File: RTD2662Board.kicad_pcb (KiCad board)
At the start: 2 copper layers, 100 x 70 mm, 263 parts, among them J1 DVI, J10 UART/I2C, J11 LCD Connector, J12 SPDIFF, J13 3.5mm jack, J14 DC Jack, J15 Expansion Connector, J2 HDMI A, J3 3.5mm jack, J4 VGA, J5 CVBS1, J6 CVBS2, J7 Mini-DIN-4, J8 USB B, J9 Keyboard Connector, Q1 BC846, Q2 BC846, Q3 AO3401A, Q4 BC846, Q5 AO3401A, SW1 POWER, SW2 MENU, SW3 UP, SW4 DOWN, SW5 SOURCE, U1 RTD2662, U10 25x128, U11 APW7313, U12 AMS1117-1.8, U2 TPS61040DBV, U3 TL1838, U4 CH341T, U5 TPS61040DBV, U6 ES7134S, U7 PAM8003, U8 TPS61040DBV, U9 24x01, Y1 27MHz, Y2 12MHz

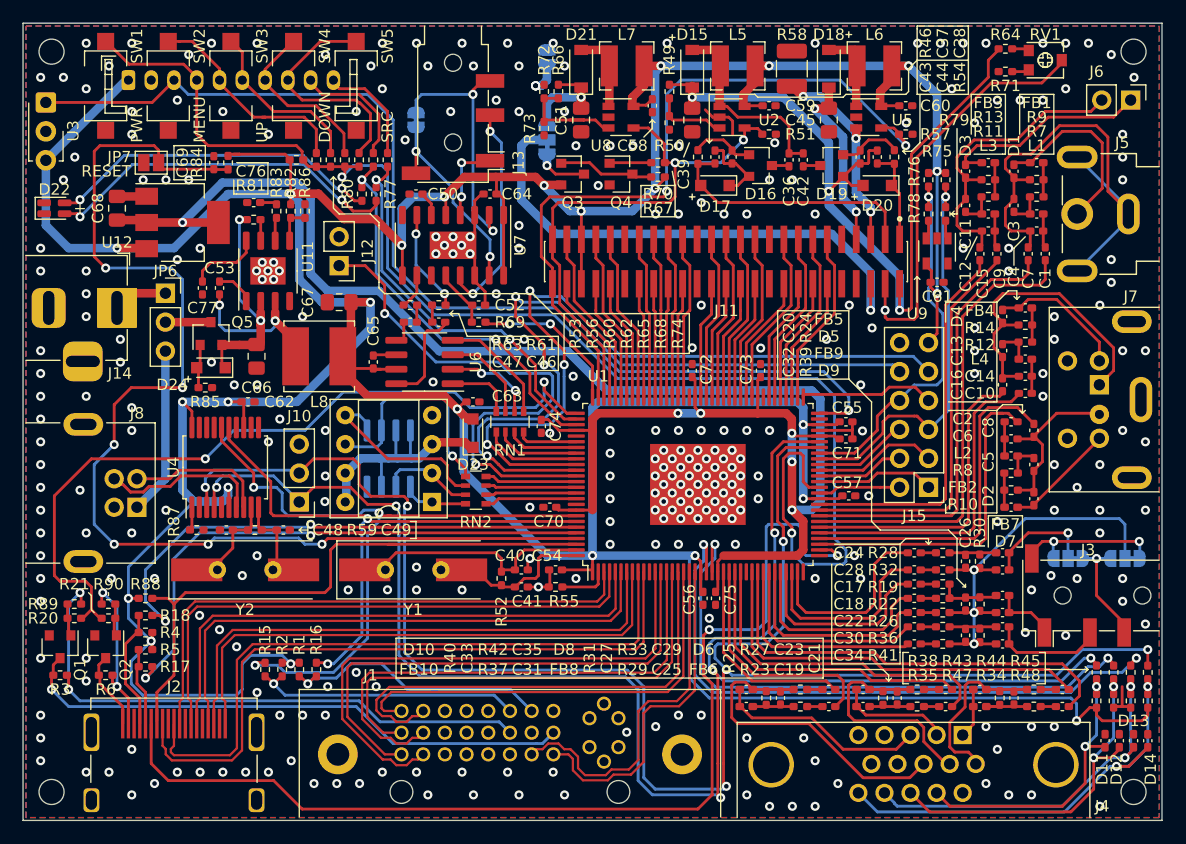
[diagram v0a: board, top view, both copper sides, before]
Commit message: KiCad version update
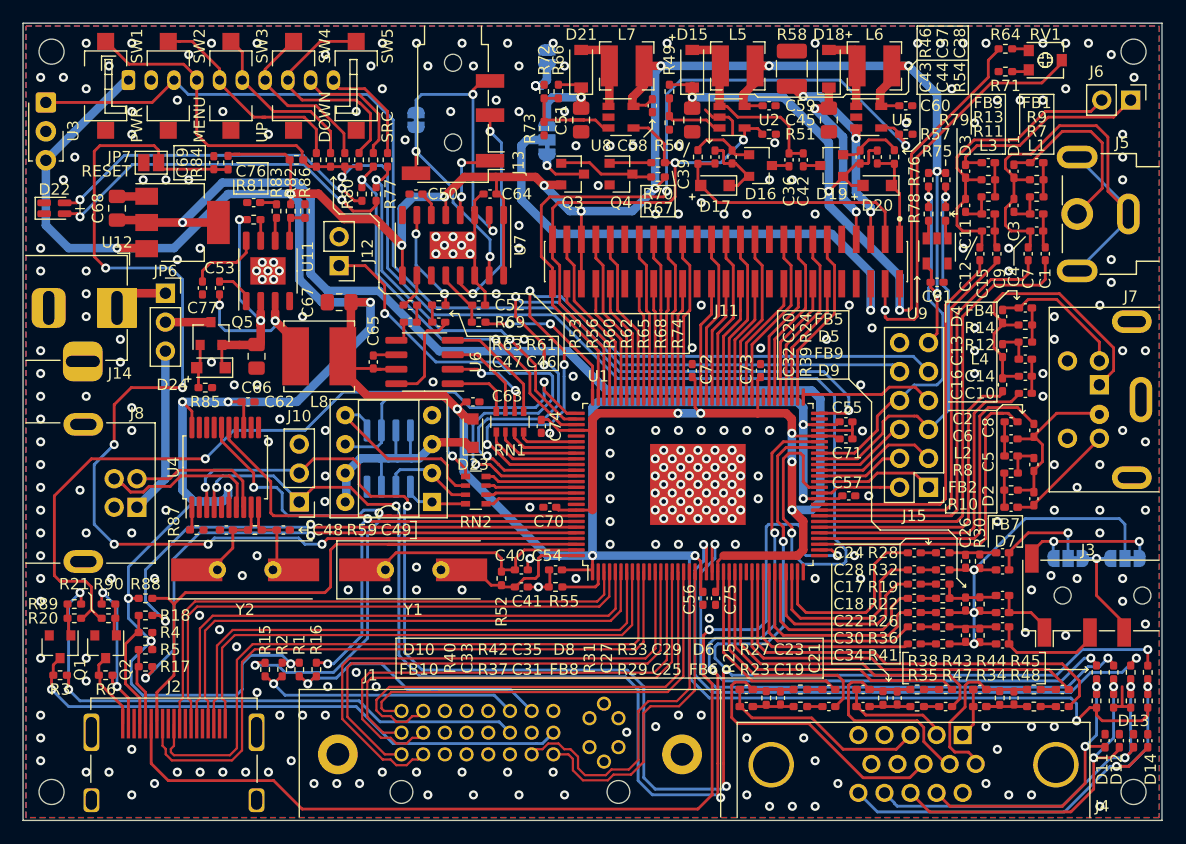
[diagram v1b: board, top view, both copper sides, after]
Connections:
- net ~RESET~ renamed ~{RESET}
- net ~SPI_CE~ renamed ~{SPI_CE}
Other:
- net class Default removed
- net class Power removed
